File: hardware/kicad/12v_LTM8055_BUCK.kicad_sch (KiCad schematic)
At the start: 20 parts, among them U44 MCP4725A0T-E/CH, U47 LTM8055IY_PBF

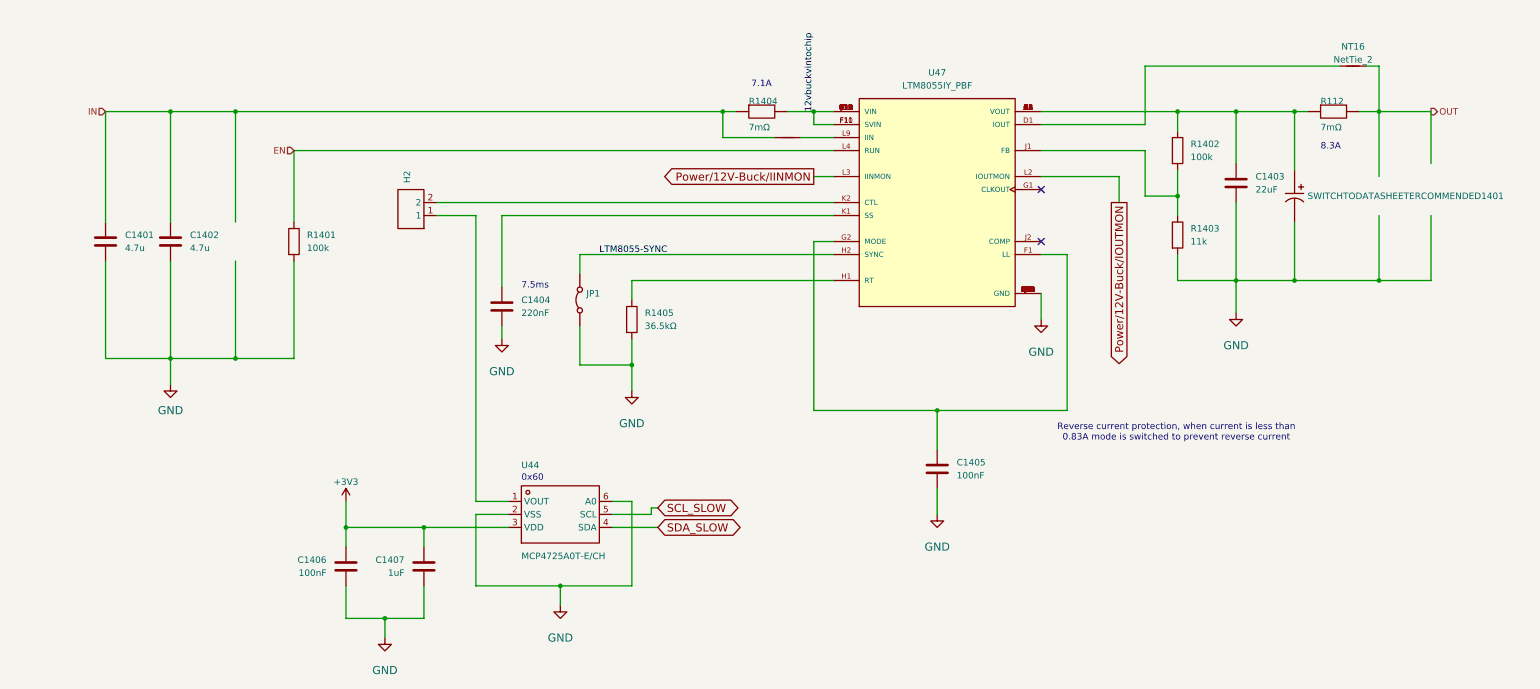
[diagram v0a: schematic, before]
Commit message: various updates
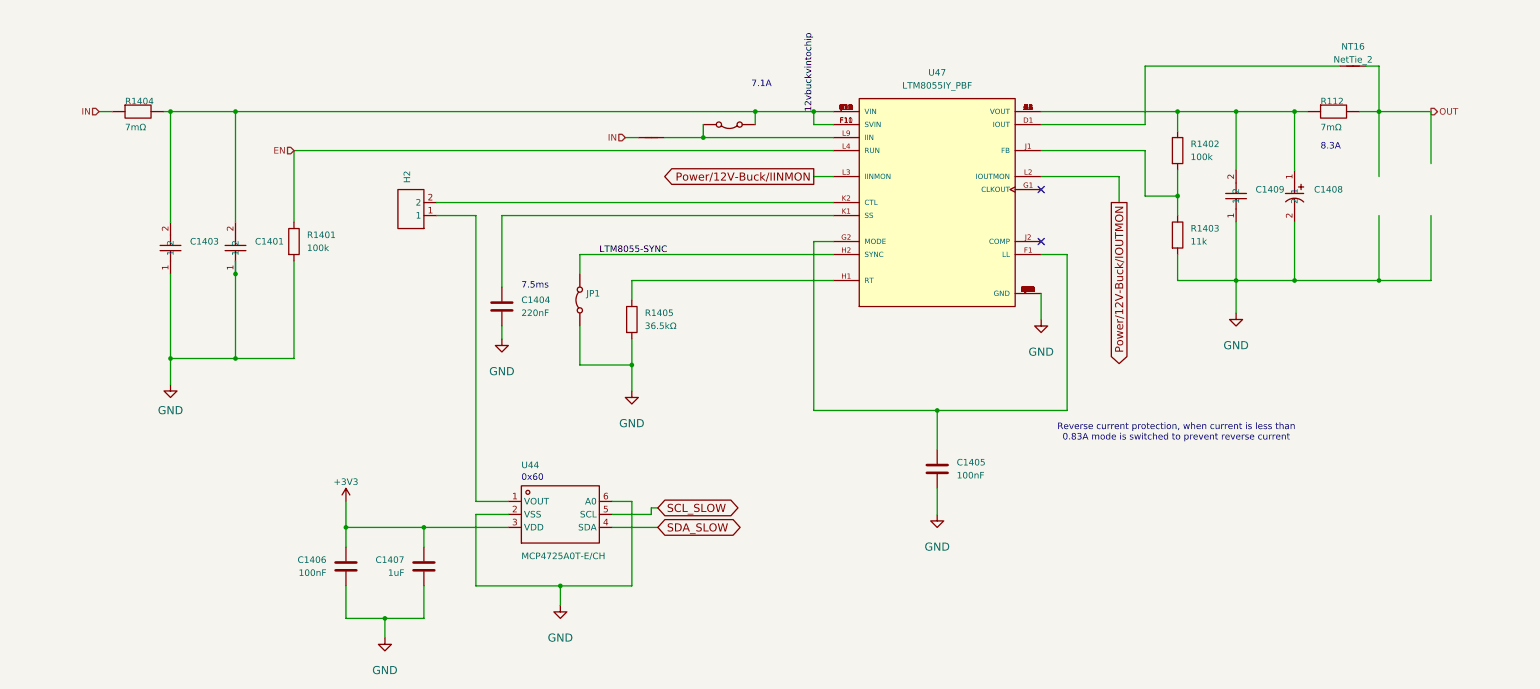
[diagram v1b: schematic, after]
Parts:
- removed C1401, C1402: 4.7u, Capacitor_SMD:C_1210_3225Metric, symbol Device:C
- removed C1403: 22uF, Capacitor_SMD:C_0805_2012Metric, symbol Device:C
- removed SWITCHTODATASHEETERCOMMENDED1401: 68uF, 5v rail sm-easyedapro:CAP-SMD_BD6.3-L6.6-W6.6-LS7.4-FD, symbol 5v rail sm-easyedapro:RVT1E680M0605
- added C1401, C1403: CL32B475KBUYNNE, JLCImport:CL32B475KBUYNNE, symbol JLCImport:CL32B475KBUYNNE
- added C1408: TPSC686M016R0200, JLCImport:TPSC686M016R0200, symbol JLCImport:TPSC686M016R0200
- added C1409: CL21A226MAYNNNE, JLCImport:CL21A226MAYNNNE, symbol JLCImport:CL21A226MAYNNNE
- added JP1401: Jumper_2_Bridged, PCM_SparkFun-Jumper:Jumper_2_NC_Trace, symbol Jumper:Jumper_2_Bridged
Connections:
- net 12vbuckvintochip: now also C1401.2, C1403.2, JP1401.1 (A)
- net GND: now also C1401.1, C1403.1, C1408.2, C1409.1
- net at R112.1, R1402.1, U47.A1 (VOUT)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: now also C1408.1, C1409.2
- net at NT1401.2, U47.L9 (IIN): now also JP1401.2 (B)
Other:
- moved on the sheet: R1404

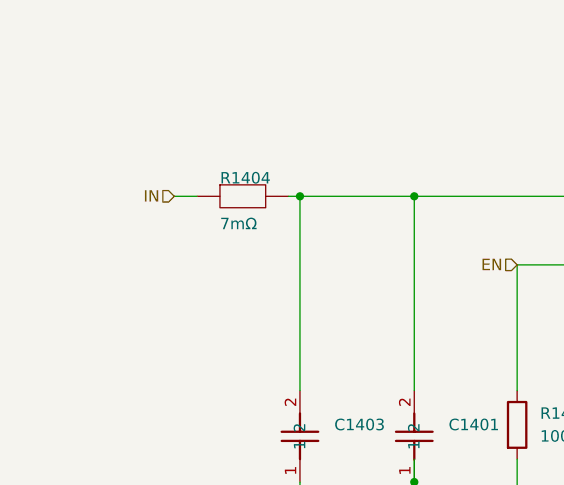
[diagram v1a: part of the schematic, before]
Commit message: various updates
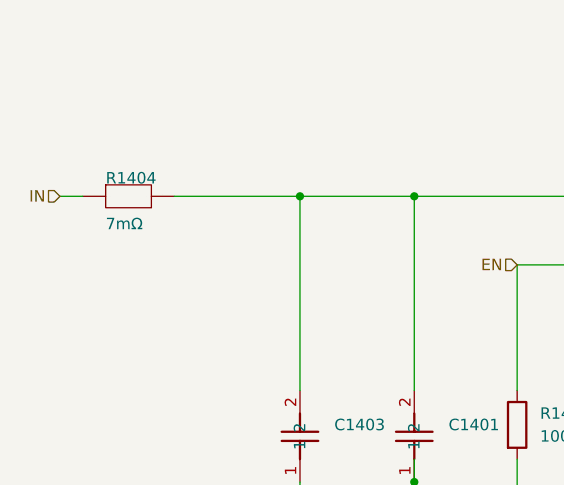
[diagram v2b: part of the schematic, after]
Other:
- moved on the sheet: R1404
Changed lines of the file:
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@@
 	(wire
 		(pts
-			(xy 16.51 66.04) (xy 19.05 66.04)
+			(xy 3.81 66.04) (xy 6.35 66.04)
 		)
 		(stroke
@@
 	(wire
 		(pts
-			(xy 29.21 66.04) (xy 30.48 66.04)
+			(xy 16.51 66.04) (xy 30.48 66.04)
 		)
 		(stroke
@@
 	(hierarchical_label "IN"
 		(shape input)
-		(at 16.51 66.04 180)
+		(at 3.81 66.04 180)
 		(effects
 			(font
@@
 	(symbol
 		(lib_id "5v rail sm-easyedapro:JER2512F3R007")
-		(at 24.13 66.04 0)
+		(at 11.43 66.04 0)
 		(unit 1)
 		(exclude_from_sim no)
@@
 		(dnp no)
 		(property "Reference" "R1404"
-			(at 21.59 64.77 0)
+			(at 8.89 64.77 0)
 			(effects
 				(font
@@
 		)
 		(property "Value" "7mΩ"
-			(at 21.59 69.85 0)
+			(at 8.89 69.85 0)
 			(effects
 				(font
@@
 		)
 		(property "Footprint" "5v rail sm-easyedapro:R2512"
-			(at 24.13 66.04 0)
+			(at 11.43 66.04 0)
 			(effects
 				(font
@@
 		)
 		(property "Datasheet" "https://item.szlcsc.com/datasheet/JER2512F3R007/51553032.html"
-			(at 24.13 66.04 0)
+			(at 11.43 66.04 0)
 			(effects
 				(font
@@
 		)
 		(property "Description" "Type:Current Sense Resistor Resistance:7mΩ Tolerance:±1% Tolerance:±1% Power(Watts):3W Temperature Coefficient:±50ppm/°C Temperature Coefficient:±50ppm/°C"
-			(at 24.13 66.04 0)
+			(at 11.43 66.04 0)
 			(effects
 				(font
@@
 		)
 		(property "Manufacturer Part" "JER2512F3R007"
-			(at 24.13 66.04 0)
+			(at 11.43 66.04 0)
 			(effects
 				(font
@@
 		)
 		(property "Manufacturer" "JIERR(捷而瑞)"
-			(at 24.13 66.04 0)
+			(at 11.43 66.04 0)
 			(effects
 				(font
@@
 		)
 		(property "Supplier Part" "C49164689"
-			(at 24.13 66.04 0)
+			(at 11.43 66.04 0)
 			(effects
 				(font
@@
 		)
 		(property "Supplier" "LCSC"
-			(at 24.13 66.04 0)
+			(at 11.43 66.04 0)
 			(effects
 				(font
@@
 		)
 		(property "LCSC Part Name" "7mΩ 3W 2512 ±1%"
-			(at 24.13 66.04 0)
-			(effects
-				(font
+			(at 11.43 66.04 0)
+			(effects
+				(font
